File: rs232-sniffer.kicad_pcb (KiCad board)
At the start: 2 copper layers, 110 x 55 mm, 78 parts, among them J1 Stiftleiste 2x8, J2 DB9_Female, J3 DB9_Male, J4 DB9_Female, J5 DB9_Female

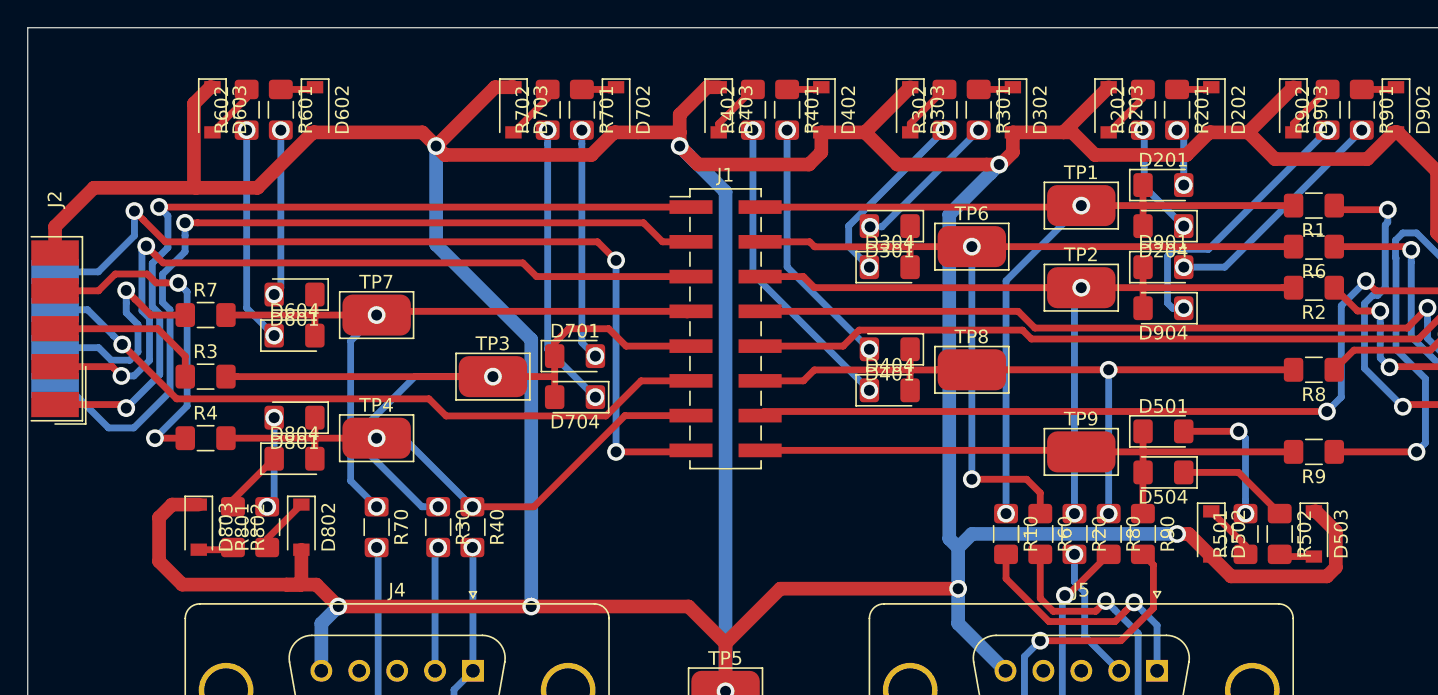
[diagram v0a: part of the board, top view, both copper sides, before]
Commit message: version marius wasinger
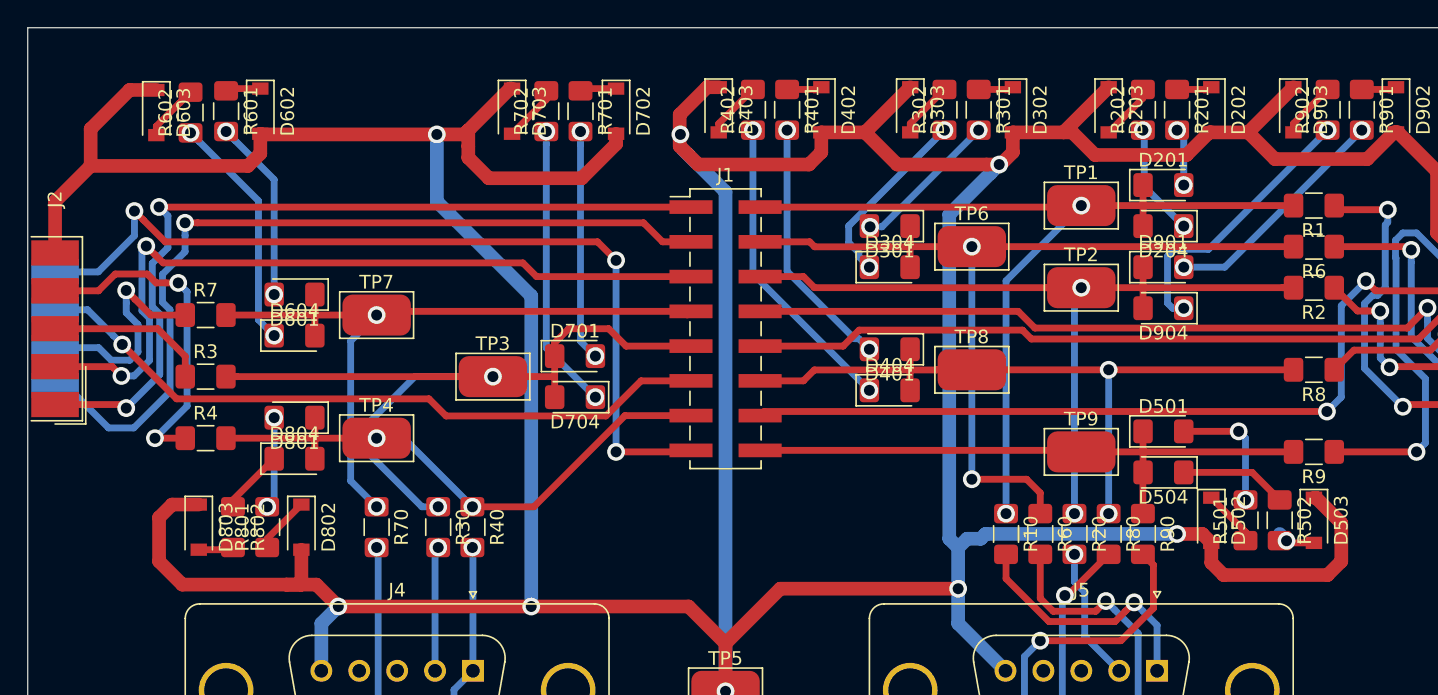
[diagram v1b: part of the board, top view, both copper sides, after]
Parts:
- J2: footprint Connector_Dsub:DSUB-9_Female_EdgeMount_P2.77mm -> rs232-sniffer:DSUB-9_Female_EdgeMount_P2.77mm
- J3: footprint Connector_Dsub:DSUB-9_Male_EdgeMount_P2.77mm -> rs232-sniffer:DSUB-9_Male_EdgeMount_P2.77mm
- J4, J5: footprint Connector_Dsub:DSUB-9_Female_Vertical_P2.77x2.84mm_MountingHoles -> rs232-sniffer:DSUB-9_Female_Vertical_P2.77x2.84mm_MountingHoles
- TP1, TP2, TP3, TP4, TP5, TP6, TP7, TP8, TP9: footprint rs232-sniffer:TestPoint_Pad_5.0x3.0mm -> rs232-sniffer:TestPoint_Pad_5.0x3.0mm_paste
- moved D603 4.10 mm to (68.4, 99.2)
- moved R602 4.10 mm to (70.9, 99.2)
- moved D602 4.00 mm to (76.0, 99.1)
- moved R601 4.00 mm to (73.5, 99.1)
- moved D502 1.00 mm to (145.5, 129.0)
- moved D503 1.00 mm to (153.0, 129.0)
- moved R501 1.00 mm to (148.0, 129.0)
- moved R502 1.00 mm to (150.5, 129.0)
- moved D703 0.14 mm to (94.4, 99.1)
- moved R701 0.14 mm to (99.4, 99.1)
- moved R702 0.14 mm to (96.9, 99.1)
- moved D702 0.10 mm to (102.0, 99.1)
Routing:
- net Net-(D604-Pad1): track 15.8 -> 17.3 mm
- net Net-(D601-Pad2): track 12.2 -> 13.4 mm
- net Net-(D501-Pad2): track 10.2 -> 9.23 mm
- net GND: track 396.0 -> 396.8 mm
- net Net-(D503-Pad2): track 2.57 -> 3.27 mm, vias 0 -> 1

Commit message: wip
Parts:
- removed D201, D301: grün, LED_SMD:LED_1206_3216Metric_Pad1.42x1.75mm_HandSolder
- removed D202, D203, D302, D303, D402, D403, D502, D503, D602, D603, D702, D703, D802, D803, D902, D903: 1N4148W, Diode_SMD:D_SOD-123
- removed D204, D304, D404, D504, D604, D704, D804, D904: rot, LED_SMD:LED_1206_3216Metric_Pad1.42x1.75mm_HandSolder
- removed J4, J5: DB9_Female, rs232-sniffer:DSUB-9_Female_Vertical_P2.77x2.84mm_MountingHoles
- removed R201, R202, R301, R302, R402, R502, R602, R702, R802, R902: 4k7, Resistor_SMD:R_1206_3216Metric_Pad1.42x1.75mm_HandSolder
- removed TP1, TP2, TP3, TP4, TP6, TP7, TP8, TP9: SMD Testpoint, rs232-sniffer:TestPoint_Pad_5.0x3.0mm_paste
- added C2101: 100n, Capacitor_SMD:C_0603_1608Metric, F.Cu at (283.8, 48.0)
- added C2102: 100n, Capacitor_SMD:C_0603_1608Metric, F.Cu at (263.8, 58.0)
- added C2201: 100n, Capacitor_SMD:C_0603_1608Metric, F.Cu at (263.8, 82.3)
- added C2202: 100n, Capacitor_SMD:C_0603_1608Metric, F.Cu at (263.8, 84.8)
- added C2203: 100n, Capacitor_SMD:C_0603_1608Metric, F.Cu at (267.8, 82.3)
- added C2204: 100n, Capacitor_SMD:C_0603_1608Metric, F.Cu at (267.8, 84.8)
- added C2205: 100n, Capacitor_SMD:C_0603_1608Metric, F.Cu at (271.8, 82.3)
- added C2301: 100n, Capacitor_SMD:C_0603_1608Metric, F.Cu at (291.9, 60.6)
- added C2302: 100n, Capacitor_SMD:C_0603_1608Metric, F.Cu at (295.9, 58.1)
- added C2303: 100n, Capacitor_SMD:C_0603_1608Metric, F.Cu at (295.9, 60.6)
- added C2304: 100n, Capacitor_SMD:C_0603_1608Metric, F.Cu at (291.9, 58.1)
- added C2305: 100n, Capacitor_SMD:C_0603_1608Metric, F.Cu at (299.9, 58.1)
- added C2501: 100n, Capacitor_SMD:C_0603_1608Metric, F.Cu at (267.8, 76.6)
- added C2502: 100n, Capacitor_SMD:C_0603_1608Metric, F.Cu at (283.8, 65.1)
- added C2601: 100n, Capacitor_SMD:C_0603_1608Metric, F.Cu at (241.3, 104.7)
- added C2602: 100n, Capacitor_SMD:C_0603_1608Metric, F.Cu at (237.3, 107.2)
- added C2603: 100n, Capacitor_SMD:C_0603_1608Metric, F.Cu at (237.3, 104.7)
- added C2604: 100n, Capacitor_SMD:C_0603_1608Metric, F.Cu at (233.3, 107.2)
- added C2605: 100n, Capacitor_SMD:C_0603_1608Metric, F.Cu at (233.3, 104.7)
- added C2701: 100n, Capacitor_SMD:C_0603_1608Metric, F.Cu at (299.9, 48.0)
- added C2702: 100n, Capacitor_SMD:C_0603_1608Metric, F.Cu at (295.9, 50.5)
- added C2703: 100n, Capacitor_SMD:C_0603_1608Metric, F.Cu at (295.9, 48.0)
- added C2704: 100n, Capacitor_SMD:C_0603_1608Metric, F.Cu at (291.9, 50.5)
- added C2705: 100n, Capacitor_SMD:C_0603_1608Metric, F.Cu at (291.9, 48.0)
- added D1001: red/green, rs232-sniffer:LED_LiteOn_LTST-C195KGJRKT, F.Cu at (298.4, 95.0)
- added D1101: red/green, rs232-sniffer:LED_LiteOn_LTST-C195KGJRKT, F.Cu at (283.6, 105.1)
- added D1301: red/green, rs232-sniffer:LED_LiteOn_LTST-C195KGJRKT, F.Cu at (312.5, 70.4)
- added D1401: red/green, rs232-sniffer:LED_LiteOn_LTST-C195KGJRKT, F.Cu at (299.2, 80.9)
- added D1501: red/green, rs232-sniffer:LED_LiteOn_LTST-C195KGJRKT, F.Cu at (268.8, 95.5)
- added D1601: red/green, rs232-sniffer:LED_LiteOn_LTST-C195KGJRKT, F.Cu at (268.8, 105.1)
- added D1701: red/green, rs232-sniffer:LED_LiteOn_LTST-C195KGJRKT, F.Cu at (312.5, 60.7)
- added D1801: red/green, rs232-sniffer:LED_LiteOn_LTST-C195KGJRKT, F.Cu at (296.9, 71.3)
- added D1901: red/green, rs232-sniffer:LED_LiteOn_LTST-C195KGJRKT, F.Cu at (284.4, 85.4)
- added D2001: red/green, rs232-sniffer:LED_LiteOn_LTST-C195KGJRKT, F.Cu at (312.5, 51.1)
- added H101: MountingHole, MountingHole:MountingHole_4mm, F.Cu at (64.0, 143.0)
- added H102: MountingHole, MountingHole:MountingHole_4mm, F.Cu at (164.0, 143.0)
- added H103: MountingHole, MountingHole:MountingHole_4mm, F.Cu at (64.0, 98.0)
- added H104: MountingHole, MountingHole:MountingHole_4mm, F.Cu at (164.0, 98.0)
- added J2101: USB-C/16p, rs232-sniffer:USB_C_Receptacle_LCSC_C167321, F.Cu at (267.6, 50.9)
- added J2501: USB-C/16p, rs232-sniffer:USB_C_Receptacle_LCSC_C167321, F.Cu at (267.6, 68.0)
- added R1001: 4k7, Resistor_SMD:R_0603_1608Metric, F.Cu at (299.0, 91.9)
- added R107: 100R, Resistor_SMD:R_0603_1608Metric, F.Cu at (223.8, 107.2)
- added R108: 100R, Resistor_SMD:R_0603_1608Metric, F.Cu at (219.8, 109.7)
- added R109: 100R, Resistor_SMD:R_0603_1608Metric, F.Cu at (223.8, 104.7)
- added R110: 100R, Resistor_SMD:R_0603_1608Metric, F.Cu at (219.8, 107.2)
- added R1101: 4k7, Resistor_SMD:R_0603_1608Metric, F.Cu at (284.2, 102.0)
- added R111: 100R, Resistor_SMD:R_0603_1608Metric, F.Cu at (215.8, 109.7)
- added R117: 100R, Resistor_SMD:R_0603_1608Metric, F.Cu at (219.8, 104.7)
- added R118: 100R, Resistor_SMD:R_0603_1608Metric, F.Cu at (215.8, 107.2)
- added R119: 100R, Resistor_SMD:R_0603_1608Metric, F.Cu at (215.8, 104.7)
- added R1301: 4k7, Resistor_SMD:R_0603_1608Metric, F.Cu at (313.1, 67.3)
- added R1401: 4k7, Resistor_SMD:R_0603_1608Metric, F.Cu at (299.8, 77.8)
- added R1501: 4k7, Resistor_SMD:R_0603_1608Metric, F.Cu at (269.4, 92.4)
- added R1601: 4k7, Resistor_SMD:R_0603_1608Metric, F.Cu at (269.4, 102.0)
- added R1701: 4k7, Resistor_SMD:R_0603_1608Metric, F.Cu at (313.1, 57.6)
- added R1801: 4k7, Resistor_SMD:R_0603_1608Metric, F.Cu at (297.5, 68.2)
- added R1901: 4k7, Resistor_SMD:R_0603_1608Metric, F.Cu at (285.0, 82.3)
- added R2001: 4k7, Resistor_SMD:R_0603_1608Metric, F.Cu at (313.1, 48.0)
- added R2101: 100R, Resistor_SMD:R_0603_1608Metric, F.Cu at (267.8, 59.5)
- added R2501: 100R, Resistor_SMD:R_0603_1608Metric, F.Cu at (263.8, 75.1)
- added SW2001: DIP-Switch 8, Button_Switch_SMD:SW_DIP_SPSTx08_Slide_6.7x21.88mm_W8.61mm_P2.54mm_LowProfile, F.Cu at (220.1, 58.6)
- added SW2401: DIP-Switch 8, Button_Switch_SMD:SW_DIP_SPSTx08_Slide_6.7x21.88mm_W8.61mm_P2.54mm_LowProfile, F.Cu at (220.1, 86.9)
- added TP1001: SMD Testpoint, rs232-sniffer:Keystone_5016, F.Cu at (294.1, 92.7)
- added TP102: SMD Testpoint, rs232-sniffer:Keystone_5016, F.Cu at (84.2, 100.8)
- added TP103: SMD Testpoint, rs232-sniffer:Keystone_5016, F.Cu at (120.2, 99.4)
- added TP1101: SMD Testpoint, rs232-sniffer:Keystone_5016, F.Cu at (279.3, 102.8)
- added TP1301: SMD Testpoint, rs232-sniffer:Keystone_5016, F.Cu at (308.2, 68.1)
- added TP1401: SMD Testpoint, rs232-sniffer:Keystone_5016, F.Cu at (294.9, 78.6)
- added TP1501: SMD Testpoint, rs232-sniffer:Keystone_5016, F.Cu at (264.5, 93.2)
- added TP1601: SMD Testpoint, rs232-sniffer:Keystone_5016, F.Cu at (264.5, 102.8)
- added TP1701: SMD Testpoint, rs232-sniffer:Keystone_5016, F.Cu at (308.2, 58.4)
- added TP1801: SMD Testpoint, rs232-sniffer:Keystone_5016, F.Cu at (292.6, 69.0)
- added TP1901: SMD Testpoint, rs232-sniffer:Keystone_5016, F.Cu at (280.1, 83.1)
- added TP2001: SMD Testpoint, rs232-sniffer:Keystone_5016, F.Cu at (308.2, 48.8)
- added TP401: SMD Testpoint, rs232-sniffer:Keystone_5016, F.Cu at (249.6, 105.5)
- added TP501: SMD Testpoint, rs232-sniffer:Keystone_5016, F.Cu at (279.3, 93.2)
- added TP601: SMD Testpoint, rs232-sniffer:Keystone_5016, F.Cu at (308.9, 97.9)
- added TP701: SMD Testpoint, rs232-sniffer:Keystone_5016, F.Cu at (308.9, 88.3)
- added TP801: SMD Testpoint, rs232-sniffer:Keystone_5016, F.Cu at (294.1, 102.4)
- added TP901: SMD Testpoint, rs232-sniffer:Keystone_5016, F.Cu at (309.7, 77.7)
- added U2101: CH340C, Package_SO:SOIC-16_3.9x9.9mm_P1.27mm, F.Cu at (277.6, 52.5)
- added U2501: CH340C, Package_SO:SOIC-16_3.9x9.9mm_P1.27mm, F.Cu at (277.6, 69.6)
- D401, D501, D601, D701, D801, D901: value grün -> red/green; footprint LED_SMD:LED_1206_3216Metric_Pad1.42x1.75mm_HandSolder -> rs232-sniffer:LED_LiteOn_LTST-C195KGJRKT
- J101: renamed from J2; footprint rs232-sniffer:DSUB-9_Female_EdgeMount_P2.77mm -> rs232-sniffer:DSUB-9_Female_Vertical_P2.77x2.84mm_MountingHoles
- R101: renamed from R7; value 0R -> 100R; footprint Resistor_SMD:R_1206_3216Metric_Pad1.42x1.75mm_HandSolder -> Resistor_SMD:R_0603_1608Metric
- R102: renamed from R3; value 0R -> 100R; footprint Resistor_SMD:R_1206_3216Metric_Pad1.42x1.75mm_HandSolder -> Resistor_SMD:R_0603_1608Metric
- R103: renamed from R4; value 0R -> 100R; footprint Resistor_SMD:R_1206_3216Metric_Pad1.42x1.75mm_HandSolder -> Resistor_SMD:R_0603_1608Metric
- R104: renamed from R70; value 0R -> 100R; footprint Resistor_SMD:R_1206_3216Metric_Pad1.42x1.75mm_HandSolder -> Resistor_SMD:R_0603_1608Metric
- R105: renamed from R30; value 0R -> 100R; footprint Resistor_SMD:R_1206_3216Metric_Pad1.42x1.75mm_HandSolder -> Resistor_SMD:R_0603_1608Metric
- R106: renamed from R40; value 0R -> 100R; footprint Resistor_SMD:R_1206_3216Metric_Pad1.42x1.75mm_HandSolder -> Resistor_SMD:R_0603_1608Metric
- R112: renamed from R10; value 0R -> 100R; footprint Resistor_SMD:R_1206_3216Metric_Pad1.42x1.75mm_HandSolder -> Resistor_SMD:R_0603_1608Metric
- R113: renamed from R60; value 0R -> 100R; footprint Resistor_SMD:R_1206_3216Metric_Pad1.42x1.75mm_HandSolder -> Resistor_SMD:R_0603_1608Metric
- R114: renamed from R20; value 0R -> 100R; footprint Resistor_SMD:R_1206_3216Metric_Pad1.42x1.75mm_HandSolder -> Resistor_SMD:R_0603_1608Metric
- R115: renamed from R80; value 0R -> 100R; footprint Resistor_SMD:R_1206_3216Metric_Pad1.42x1.75mm_HandSolder -> Resistor_SMD:R_0603_1608Metric
- R116: renamed from R90; value 0R -> 100R; footprint Resistor_SMD:R_1206_3216Metric_Pad1.42x1.75mm_HandSolder -> Resistor_SMD:R_0603_1608Metric
- R120: renamed from R1; value 0R -> 100R; footprint Resistor_SMD:R_1206_3216Metric_Pad1.42x1.75mm_HandSolder -> Resistor_SMD:R_0603_1608Metric
- R121: renamed from R6; value 0R -> 100R; footprint Resistor_SMD:R_1206_3216Metric_Pad1.42x1.75mm_HandSolder -> Resistor_SMD:R_0603_1608Metric
- R122: renamed from R2; value 0R -> 100R; footprint Resistor_SMD:R_1206_3216Metric_Pad1.42x1.75mm_HandSolder -> Resistor_SMD:R_0603_1608Metric
- R123: renamed from R8; value 0R -> 100R; footprint Resistor_SMD:R_1206_3216Metric_Pad1.42x1.75mm_HandSolder -> Resistor_SMD:R_0603_1608Metric
- R124: renamed from R9; value 0R -> 100R; footprint Resistor_SMD:R_1206_3216Metric_Pad1.42x1.75mm_HandSolder -> Resistor_SMD:R_0603_1608Metric
- R401, R501, R601, R701, R801, R901: footprint Resistor_SMD:R_1206_3216Metric_Pad1.42x1.75mm_HandSolder -> Resistor_SMD:R_0603_1608Metric
- TP101: renamed from TP5; footprint rs232-sniffer:TestPoint_Pad_5.0x3.0mm_paste -> rs232-sniffer:Keystone_5016
- moved R601 240.3 mm to (313.8, 97.1), turned to 0 degrees
- moved D601 235.1 mm to (313.2, 100.2), turned to 0 degrees
- moved R801 224.2 mm to (299.0, 101.6), turned to 0 degrees
- moved D801 220.6 mm to (298.4, 104.6), turned to 0 degrees
- moved D701 215.9 mm to (313.2, 90.6)
- moved R701 214.7 mm to (313.8, 87.5), turned to 0 degrees
- moved D901 174.7 mm to (314.0, 80.0)
- moved R901 159.6 mm to (314.6, 76.9), turned to 0 degrees
- moved D501 144.2 mm to (283.6, 95.5)
- moved R501 141.0 mm to (284.2, 92.4), turned to 0 degrees
- moved R401 140.1 mm to (254.5, 104.7), turned to 0 degrees
- moved D401 132.2 mm to (253.9, 107.7), turned to 0 degrees
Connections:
- D401 pad 1: /ClearToSend -> Net-(D401-Pad1)
- D401 pad 2: Net-(D401-Pad2) -> /LEDs A/Signal1
- D501 pad 1: /RingIndicator -> Net-(D501-Pad1)
- D501 pad 2: Net-(D501-Pad2) -> /LEDs A/Signal2
- D601 pad 1: /ReadyToReceive -> Net-(D601-Pad1)
- D601 pad 2: Net-(D601-Pad2) -> /LEDs A/Signal3
- D701 pad 1: /Sig3 -> Net-(D701-Pad1)
- D701 pad 2: Net-(D701-Pad2) -> /LEDs A/Signal4
- D801 pad 1: /DataTerminalReady -> Net-(D801-Pad1)
- D801 pad 2: Net-(D801-Pad2) -> /LEDs A/Signal6
- D901 pad 1: /ReceiveData -> Net-(D901-Pad1)
- D901 pad 2: Net-(D901-Pad2) -> /LEDs A/Signal7
- J1 pad 1: Net-(J1-Pad1) -> (no net)
- J1 pad 11: /ClearToSend -> (no net)
- J1 pad 14: /ReceiveData -> (no net)
- J1 pad 15: /DataSetReady -> (no net)
- J1 pad 16: /DataCarrierDetect -> (no net)
- J1 pad 2: Net-(J1-Pad2) -> (no net)
- J1 pad 3: Net-(J1-Pad3) -> (no net)
- J1 pad 4: /ReadyToReceive -> (no net)
- J1 pad 5: /Sig3 -> (no net)
- J1 pad 6: Net-(J1-Pad6) -> (no net)
- J1 pad 7: /DataTerminalReady -> (no net)
- J1 pad 8: Net-(J1-Pad8) -> (no net)
- J1 pad 9: /RingIndicator -> (no net)
- J101 pad 1: Net-(J1-Pad1) -> /LEDs A/Signal1
- J101 pad 2: Net-(J1-Pad3) -> /LEDs A/Signal2
- J101 pad 6: Net-(J1-Pad2) -> /LEDs A/Signal6
- J101 pad 8: Net-(J1-Pad6) -> /LEDs A/Signal8
- J101 pad 9: Net-(J1-Pad8) -> /LEDs A/Signal9
- J3 pad 1: Net-(J3-Pad1) -> (no net)
- J3 pad 2: Net-(J3-Pad2) -> (no net)
- J3 pad 6: Net-(J3-Pad6) -> (no net)
- J3 pad 8: Net-(J3-Pad8) -> (no net)
- J3 pad 9: Net-(J3-Pad9) -> (no net)
- R101 pad 2: /ReadyToReceive -> /LEDs A/Signal7
- R102 pad 2: /Sig3 -> /LEDs A/Signal3
- R103 pad 2: /DataTerminalReady -> /LEDs A/Signal4
- R104 pad 1: /ReadyToReceive -> /LEDs A/Signal7
- R104 pad 2: Net-(J4-Pad8) -> (no net)
- R105 pad 1: /Sig3 -> /LEDs A/Signal3
- R105 pad 2: Net-(J4-Pad2) -> (no net)
- R106 pad 1: /DataTerminalReady -> /LEDs A/Signal4
- R106 pad 2: Net-(J4-Pad1) -> (no net)
- R112 pad 1: /DataCarrierDetect -> /LEDs B/Signal1
- R112 pad 2: Net-(J5-Pad1) -> (no net)
- R113 pad 1: /DataSetReady -> /LEDs B/Signal6
- R113 pad 2: Net-(J5-Pad6) -> (no net)
- R114 pad 1: /ReceiveData -> /LEDs B/Signal2
- R114 pad 2: Net-(J5-Pad2) -> (no net)
- R115 pad 1: /ClearToSend -> /LEDs B/Signal8
- R115 pad 2: Net-(J5-Pad8) -> (no net)
- R116 pad 1: /RingIndicator -> /LEDs B/Signal9
- R116 pad 2: Net-(J5-Pad9) -> (no net)
- R120 pad 1: Net-(J3-Pad1) -> (no net)
- R120 pad 2: /DataCarrierDetect -> /LEDs B/Signal1
- R121 pad 1: Net-(J3-Pad6) -> (no net)
- R121 pad 2: /DataSetReady -> /LEDs B/Signal6
- R122 pad 1: Net-(J3-Pad2) -> (no net)
- R122 pad 2: /ReceiveData -> /LEDs B/Signal2
- R123 pad 1: Net-(J3-Pad8) -> (no net)
- R123 pad 2: /ClearToSend -> /LEDs B/Signal8
- R124 pad 1: Net-(J3-Pad9) -> (no net)
- R124 pad 2: /RingIndicator -> /LEDs B/Signal9
- R401 pad 1: Net-(D402-Pad1) -> Net-(D401-Pad1)
- R401 pad 2: Net-(D401-Pad2) -> GND
- R501 pad 1: Net-(D502-Pad1) -> Net-(D501-Pad1)
- R501 pad 2: Net-(D501-Pad2) -> GND
- R601 pad 1: Net-(D602-Pad1) -> Net-(D601-Pad1)
- R601 pad 2: Net-(D601-Pad2) -> GND
- R701 pad 1: Net-(D702-Pad1) -> Net-(D701-Pad1)
- R701 pad 2: Net-(D701-Pad2) -> GND
- R801 pad 1: Net-(D802-Pad1) -> Net-(D801-Pad1)
- R801 pad 2: Net-(D801-Pad2) -> GND
- R901 pad 1: Net-(D902-Pad1) -> Net-(D901-Pad1)
- R901 pad 2: Net-(D901-Pad2) -> GND
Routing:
- net (no net): track 0.00 -> 854.3 mm, vias 0 -> 30
- net /DataCarrierDetect: track 66.8 -> 0.00 mm, vias 2 -> 0
- net /DataSetReady: track 66.1 -> 0.00 mm, vias 2 -> 0
- net Net-(J1-Pad8): track 64.9 -> 0.00 mm, vias 3 -> 0
- net /ReceiveData: track 62.5 -> 0.00 mm, vias 2 -> 0
- net Net-(J1-Pad2): track 61.7 -> 0.00 mm, vias 1 -> 0
- net Net-(J1-Pad1): track 60.9 -> 0.00 mm, vias 2 -> 0
- net /Sig3: track 58.8 -> 0.00 mm, vias 2 -> 0
- net Net-(J1-Pad3): track 57.1 -> 0.00 mm, vias 2 -> 0
- net /ReadyToReceive: track 53.1 -> 0.00 mm, vias 2 -> 0
- net /ClearToSend: track 52.8 -> 0.00 mm, vias 2 -> 0
- net Net-(J1-Pad6): track 50.8 -> 0.00 mm, vias 1 -> 0
- net /RingIndicator: track 45.2 -> 0.00 mm
- net /DataTerminalReady: track 41.8 -> 0.00 mm, vias 2 -> 0
- net Net-(J3-Pad9): track 32.1 -> 0.00 mm, vias 1 -> 0
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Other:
- outline, holes or cut-outs redrawn
- board text added: "TODO: USB-Uart"

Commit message: übergabe an 3ahel
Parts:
- removed D1101, D2001: red/green, rs232-sniffer:LED_LiteOn_LTST-C195KGJRKT
- removed J1: Stiftleiste 2x8, rs232-sniffer:PinHeader_2x08_P2.54mm_Vertical_SMD
- removed J3: DB9_Male, rs232-sniffer:DSUB-9_Male_EdgeMount_P2.77mm
- removed R1101: 4k7, Resistor_SMD:R_0603_1608Metric
- removed R121, R122, R123, R124: 100R, Resistor_SMD:R_0603_1608Metric
- removed TP1101, TP2001: SMD Testpoint, rs232-sniffer:Keystone_5016
- added C101: 10u/16V/X5R, Capacitor_SMD:C_0805_2012Metric, F.Cu at (170.5, 65.5)
- added C102: 10u/16V/X5R, Capacitor_SMD:C_0805_2012Metric, F.Cu at (174.5, 63.0)
- added C2103: 100n, Capacitor_SMD:C_0603_1608Metric, F.Cu at (100.5, 154.2)
- added C2503: 100n, Capacitor_SMD:C_0603_1608Metric, F.Cu at (20.8, 172.5)
- added D101: red/green, htl_smd:LED_LiteOn_LTST-C195KGJRKT, F.Cu at (162.5, 75.2)
- added D102: red/green, htl_smd:LED_LiteOn_LTST-C195KGJRKT, F.Cu at (159.5, 70.0)
- added D1201: red/green, htl_smd:LED_LiteOn_LTST-C195KGJRKT, F.Cu at (121.2, 42.0)
- added D301: red/green, htl_smd:LED_LiteOn_LTST-C195KGJRKT, F.Cu at (53.0, 42.1)
- added J102: Stiftleiste 2x9, Connector_PinHeader_2.54mm:PinHeader_2x09_P2.54mm_Vertical_SMD, F.Cu at (84.5, 52.0)
- added J103: DB9_Male, htl_connectors:DSUB-9_Male_EdgeMount_P2.77mm, F.Cu at (105.5, 42.0)
- added J104: Stiftleiste 2x9, Connector_PinHeader_2.54mm:PinHeader_2x09_P2.54mm_Vertical_SMD, F.Cu at (164.5, 51.5)
- added J2001: Stiftleiste 2x9, Connector_PinHeader_2.54mm:PinHeader_2x09_P2.54mm_Vertical_SMD, F.Cu at (133.0, 149.8)
- added J2002: Buchsenleiste 1x6, horizontal, Connector_PinSocket_2.54mm:PinSocket_1x06_P2.54mm_Horizontal, F.Cu at (85.0, 155.0)
- added J2003: Stiftleiste 2x9, Connector_PinHeader_2.54mm:PinHeader_2x09_P2.54mm_Vertical_SMD, F.Cu at (133.0, 115.5)
- added J2401: Stiftleiste 2x9, Connector_PinHeader_2.54mm:PinHeader_2x09_P2.54mm_Vertical_SMD, F.Cu at (53.2, 168.0)
- added J2402: Buchsenleiste 1x6, horizontal, Connector_PinSocket_2.54mm:PinSocket_1x06_P2.54mm_Horizontal, F.Cu at (72.8, 176.2)
- added J2403: Stiftleiste 2x9, Connector_PinHeader_2.54mm:PinHeader_2x09_P2.54mm_Vertical_SMD, F.Cu at (53.2, 142.8)
- added R1201: 4k7, Resistor_SMD:R_0603_1608Metric, F.Cu at (123.2, 42.0)
- added R2002: 100R, Resistor_SMD:R_0603_1608Metric, F.Cu at (124.5, 142.2)
- added R2003: 100R, Resistor_SMD:R_0603_1608Metric, F.Cu at (124.5, 144.8)
- added R2004: 1k, Resistor_SMD:R_0603_1608Metric, F.Cu at (124.5, 147.2)
- added R2005: 1k, Resistor_SMD:R_0603_1608Metric, F.Cu at (124.5, 149.8)
- added R2006: 1k, Resistor_SMD:R_0603_1608Metric, F.Cu at (124.5, 152.2)
- added R2007: 1k, Resistor_SMD:R_0603_1608Metric, F.Cu at (124.5, 154.8)
- added R2008: 1k, Resistor_SMD:R_0603_1608Metric, F.Cu at (124.5, 157.2)
- added R2009: 1k, Resistor_SMD:R_0603_1608Metric, F.Cu at (124.5, 105.2)
- added R2010: 1k, Resistor_SMD:R_0603_1608Metric, F.Cu at (124.5, 108.0)
- added R2011: 1k, Resistor_SMD:R_0603_1608Metric, F.Cu at (124.5, 110.5)
- added R2012: 100R, Resistor_SMD:R_0603_1608Metric, F.Cu at (124.5, 113.0)
- added R2013: 100R, Resistor_SMD:R_0603_1608Metric, F.Cu at (124.5, 115.5)
- added R2014: 100R, Resistor_SMD:R_0603_1608Metric, F.Cu at (124.5, 118.0)
- added R2015: 100R, Resistor_SMD:R_0603_1608Metric, F.Cu at (124.5, 120.5)
- added R2016: 100R, Resistor_SMD:R_0603_1608Metric, F.Cu at (124.5, 123.0)
- added R2401: 100R, Resistor_SMD:R_0603_1608Metric, F.Cu at (44.8, 157.8)
- added R2402: 100R, Resistor_SMD:R_0603_1608Metric, F.Cu at (44.8, 160.5)
- added R2403: 100R, Resistor_SMD:R_0603_1608Metric, F.Cu at (44.8, 163.0)
- added R2404: 1k, Resistor_SMD:R_0603_1608Metric, F.Cu at (44.8, 165.5)
- added R2405: 1k, Resistor_SMD:R_0603_1608Metric, F.Cu at (44.8, 168.0)
- added R2406: 1k, Resistor_SMD:R_0603_1608Metric, F.Cu at (44.8, 170.5)
- added R2407: 1k, Resistor_SMD:R_0603_1608Metric, F.Cu at (44.8, 173.0)
- added R2408: 1k, Resistor_SMD:R_0603_1608Metric, F.Cu at (44.8, 175.5)
- added R2409: 1k, Resistor_SMD:R_0603_1608Metric, F.Cu at (44.8, 132.5)
- added R2410: 1k, Resistor_SMD:R_0603_1608Metric, F.Cu at (44.8, 135.2)
- added R2411: 1k, Resistor_SMD:R_0603_1608Metric, F.Cu at (44.8, 137.8)
- added R2412: 100R, Resistor_SMD:R_0603_1608Metric, F.Cu at (44.8, 140.2)
- added R2413: 100R, Resistor_SMD:R_0603_1608Metric, F.Cu at (44.8, 142.8)
- added R2414: 100R, Resistor_SMD:R_0603_1608Metric, F.Cu at (44.8, 145.2)
- added R2415: 100R, Resistor_SMD:R_0603_1608Metric, F.Cu at (44.8, 147.8)
- added R2416: 100R, Resistor_SMD:R_0603_1608Metric, F.Cu at (44.8, 150.2)
- added R301: 4k7, Resistor_SMD:R_0603_1608Metric, F.Cu at (55.0, 42.1)
- added SW101: DIP-Switch 8, Button_Switch_SMD:SW_DIP_SPSTx08_Slide_6.7x21.88mm_W8.61mm_P2.54mm_LowProfile, F.Cu at (84.5, 71.0)
- added TP1201: SMD Testpoint, htl_smd:Keystone_5016, F.Cu at (117.8, 42.0)
- added TP301: SMD Testpoint, htl_smd:Keystone_5016, F.Cu at (49.5, 42.1)
- added U101: AMS1117-3.3, Package_TO_SOT_SMD:SOT-223-3_TabPin2, F.Cu at (172.2, 72.2)
- added U2201: MAX3232, Package_SO:SOIC-16_3.9x9.9mm_P1.27mm, F.Cu at (105.0, 120.0)
- added U2301: MAX3232, Package_SO:SOIC-16_3.9x9.9mm_P1.27mm, F.Cu at (115.8, 120.0)
- added U2601: MAX3232, Package_SO:SOIC-16_3.9x9.9mm_P1.27mm, F.Cu at (25.2, 136.8)
- added U2701: MAX3232, Package_SO:SOIC-16_3.9x9.9mm_P1.27mm, F.Cu at (36.0, 136.8)
- D1001, D1301, D1401, D1501, D1601, D1701, D1801, D1901, D401, D501, D601, D701, D801, D901: footprint rs232-sniffer:LED_LiteOn_LTST-C195KGJRKT -> htl_smd:LED_LiteOn_LTST-C195KGJRKT
- J101: footprint rs232-sniffer:DSUB-9_Female_Vertical_P2.77x2.84mm_MountingHoles -> htl_connectors:DSUB-9_Female_EdgeMount_P2.77mm
- J2101, J2501: footprint rs232-sniffer:USB_C_Receptacle_LCSC_C167321 -> htl_connectors:USB_C_Receptacle_LCSC_C167321
- R117, R118: value 100R -> 0R
- R119: value 100R -> 4k7
- R120: value 100R -> 1k
- R2001: value 4k7 -> 100R
- TP1001, TP101, TP102, TP103, TP1301, TP1401, TP1501, TP1601, TP1701, TP1801, TP1901, TP401, TP501, TP601, TP701, TP801, TP901: footprint rs232-sniffer:Keystone_5016 -> htl_smd:Keystone_5016
- moved C2502 284.0 mm to (23.2, 178.2), turned to 180 degrees
- moved C2701 273.9 mm to (39.0, 131.2), turned to 180 degrees
- moved C2703 272.9 mm to (36.0, 131.2), turned to 180 degrees
- moved C2702 271.9 mm to (35.0, 127.0), turned to 90 degrees
- moved U2501 271.6 mm to (26.5, 173.2), turned to 90 degrees
- moved C2704 271.2 mm to (33.0, 131.2)
- moved C2705 266.4 mm to (38.2, 129.5)
- moved D601 264.2 mm to (53.0, 54.8)
- moved TP601 263.0 mm to (49.5, 54.8)
- moved R601 262.3 mm to (55.0, 54.8), turned to 270 degrees
- moved D701 262.1 mm to (53.0, 59.1)
- moved D901 261.3 mm to (53.0, 67.6)
- moved TP701 261.1 mm to (49.5, 59.1)
- moved TP901 260.4 mm to (49.5, 67.6)
- moved R701 260.4 mm to (55.0, 59.1), turned to 270 degrees
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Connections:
- net /UART Hub/USB - UART/~CTS renamed /UART Hub R/USB - UART/~CTS
- net /UART Hub/USB - UART/~RI renamed /UART Hub R/USB - UART/~RI
- net /sheet5F8AD0D9/USB - UART/~CTS renamed /UART Hub L/USB - UART/~CTS
- net /sheet5F8AD0D9/USB - UART/~RI renamed /UART Hub L/USB - UART/~RI
- net Net-(J2101-PadA6) renamed /UART Hub R/USB - UART/D+
- net Net-(J2101-PadA7) renamed /UART Hub R/USB - UART/D-
- net Net-(J2501-PadA6) renamed /UART Hub L/USB - UART/D+
- net Net-(J2501-PadA7) renamed /UART Hub L/USB - UART/D-
- C2101 pad 1: Net-(C2101-Pad1) -> GND
- C2101 pad 2: GND -> Net-(C2101-Pad2)
- C2102 pad 1: GND -> Net-(C2102-Pad1)
- C2102 pad 2: VDD -> GND
- C2201 pad 1: (no net) -> Net-(C2201-Pad1)
- C2201 pad 2: (no net) -> Net-(C2201-Pad2)
- C2202 pad 2: VDD -> +3V3
- C2203 pad 1: (no net) -> Net-(C2203-Pad1)
- C2203 pad 2: (no net) -> Net-(C2203-Pad2)
- C2204 pad 2: (no net) -> Net-(C2204-Pad2)
- C2205 pad 2: (no net) -> Net-(C2205-Pad2)
- C2301 pad 1: (no net) -> Net-(C2301-Pad1)
- C2301 pad 2: (no net) -> Net-(C2301-Pad2)
- C2302 pad 2: VDD -> +3V3
- C2303 pad 1: (no net) -> Net-(C2303-Pad1)
- C2303 pad 2: (no net) -> Net-(C2303-Pad2)
- C2304 pad 2: (no net) -> Net-(C2304-Pad2)
- C2305 pad 2: (no net) -> Net-(C2305-Pad2)
- C2501 pad 1: Net-(C2501-Pad1) -> GND
- C2501 pad 2: GND -> Net-(C2501-Pad2)
- C2502 pad 1: GND -> Net-(C2502-Pad1)
- C2502 pad 2: VDD -> GND
- C2601 pad 1: (no net) -> Net-(C2601-Pad1)
- C2601 pad 2: (no net) -> Net-(C2601-Pad2)
- C2602 pad 2: VDD -> +3V3
- C2603 pad 1: (no net) -> Net-(C2603-Pad1)
- C2603 pad 2: (no net) -> Net-(C2603-Pad2)
- C2604 pad 2: (no net) -> Net-(C2604-Pad2)
- C2605 pad 2: (no net) -> Net-(C2605-Pad2)
- C2701 pad 1: (no net) -> Net-(C2701-Pad1)
- C2701 pad 2: (no net) -> Net-(C2701-Pad2)
- C2702 pad 2: VDD -> +3V3
- C2703 pad 1: (no net) -> Net-(C2703-Pad1)
- C2703 pad 2: (no net) -> Net-(C2703-Pad2)
- C2704 pad 2: (no net) -> Net-(C2704-Pad2)
- C2705 pad 2: (no net) -> Net-(C2705-Pad2)
- D1001 pad 2: /LEDs A/Signal8 -> GND
- D1001 pad 3: /LEDs A/Signal8 -> GND
- D1301 pad 2: /LEDs B/Signal1 -> /LEDs B/Signal2
- D1301 pad 3: /LEDs B/Signal1 -> /LEDs B/Signal2
- D1401 pad 2: /LEDs B/Signal2 -> /LEDs B/Signal3
- D1401 pad 3: /LEDs B/Signal2 -> /LEDs B/Signal3
- D1501 pad 2: /LEDs B/Signal3 -> /LEDs B/Signal4
- D1501 pad 3: /LEDs B/Signal3 -> /LEDs B/Signal4
- D1601 pad 2: /LEDs B/Signal4 -> /LEDs B/Signal6
- D1601 pad 3: /LEDs B/Signal4 -> /LEDs B/Signal6
- D1701 pad 2: /LEDs B/Signal6 -> /LEDs B/Signal7
- D1701 pad 3: /LEDs B/Signal6 -> /LEDs B/Signal7
- D1801 pad 2: /LEDs B/Signal7 -> /LEDs B/Signal8
- D1801 pad 3: /LEDs B/Signal7 -> /LEDs B/Signal8
- D1901 pad 2: /LEDs B/Signal8 -> /LEDs B/Signal9
- D1901 pad 3: /LEDs B/Signal8 -> /LEDs B/Signal9
- D401 pad 2: /LEDs A/Signal1 -> /LEDs A/Signal2
- D401 pad 3: /LEDs A/Signal1 -> /LEDs A/Signal2
- D501 pad 2: /LEDs A/Signal2 -> /LEDs A/Signal3
- D501 pad 3: /LEDs A/Signal2 -> /LEDs A/Signal3
- D601 pad 2: /LEDs A/Signal3 -> /LEDs A/Signal4
- D601 pad 3: /LEDs A/Signal3 -> /LEDs A/Signal4
- D701 pad 2: /LEDs A/Signal4 -> /LEDs A/Signal6
- D701 pad 3: /LEDs A/Signal4 -> /LEDs A/Signal6
- D801 pad 2: /LEDs A/Signal6 -> /LEDs A/Signal7
- D801 pad 3: /LEDs A/Signal6 -> /LEDs A/Signal7
- D901 pad 2: /LEDs A/Signal7 -> /LEDs A/Signal8
- D901 pad 3: /LEDs A/Signal7 -> /LEDs A/Signal8
- J101 pad 3: Net-(J101-Pad3) -> /LEDs A/Signal3
- J101 pad 4: Net-(J101-Pad4) -> /LEDs A/Signal4
- J101 pad 7: Net-(J101-Pad7) -> /LEDs A/Signal7
- J101 pad 9: /LEDs A/Signal9 -> Net-(J101-Pad9)
- J2101 pad A4: VDD -> /UART Hub R/USB-Power
- J2101 pad A9: VDD -> /UART Hub R/USB-Power
- J2101 pad B4: VDD -> /UART Hub R/USB-Power
- J2101 pad B9: VDD -> /UART Hub R/USB-Power
- J2101 pad S1: Net-(J2101-PadS1) -> Net-(C2101-Pad2)
- J2501 pad A4: VDD -> /UART Hub L/USB-Power
- J2501 pad A9: VDD -> /UART Hub L/USB-Power
- J2501 pad B4: VDD -> /UART Hub L/USB-Power
- J2501 pad B9: VDD -> /UART Hub L/USB-Power
- J2501 pad S1: Net-(J2501-PadS1) -> Net-(C2501-Pad2)
- R101 pad 1: Net-(J101-Pad7) -> /LEDs A/Signal3
- R101 pad 2: /LEDs A/Signal7 -> /UART Hub L/RxD
- R102 pad 1: Net-(J101-Pad3) -> /LEDs A/Signal4
- R102 pad 2: /LEDs A/Signal3 -> /UART Hub L/~DCD
- R103 pad 1: Net-(J101-Pad4) -> /LEDs A/Signal4
- R103 pad 2: /LEDs A/Signal4 -> /UART Hub L/~DSR
- R104 pad 2: (no net) -> /UART Hub L/~CTS
- R105 pad 1: /LEDs A/Signal3 -> /UART Hub L/TxD
- R105 pad 2: (no net) -> Net-(R105-Pad2)
- R106 pad 1: /LEDs A/Signal4 -> /UART Hub L/~DTR
- R106 pad 2: (no net) -> Net-(R106-Pad2)
- R107 pad 1: /LEDs A/Signal4 -> /UART Hub L/~DTR
- R107 pad 2: (no net) -> Net-(R107-Pad2)
- R108 pad 1: (no net) -> /UART Hub L/~RTR
- R108 pad 2: (no net) -> Net-(R108-Pad2)
- R109 pad 1: (no net) -> /UART Hub R/TxD
- R109 pad 2: (no net) -> Net-(R109-Pad2)
- R110 pad 1: /UART Hub/~DTR -> /UART Hub R/~DTR
- R110 pad 2: (no net) -> Net-(R110-Pad2)
- R111 pad 1: /UART Hub/~DTR -> /UART Hub R/~RTR
- R111 pad 2: (no net) -> Net-(R111-Pad2)
- R112 pad 1: /LEDs B/Signal1 -> /LEDs B/Signal2
- R112 pad 2: (no net) -> /UART Hub R/RxD
- R113 pad 1: /LEDs B/Signal6 -> /LEDs B/Signal1
- R113 pad 2: (no net) -> /UART Hub R/~DCD
- R114 pad 1: /LEDs B/Signal2 -> /LEDs B/Signal6
- R114 pad 2: (no net) -> /UART Hub R/~DSR
- R115 pad 2: (no net) -> /UART Hub R/~CTS
- R117 pad 1: (no net) -> /UART Hub R/USB-Power
- R117 pad 2: (no net) -> +5V
- R118 pad 1: (no net) -> /UART Hub L/USB-Power
- R118 pad 2: (no net) -> +5V
- R119 pad 1: (no net) -> +5V
- R119 pad 2: (no net) -> Net-(D101-Pad1)
- R120 pad 1: (no net) -> +3V3
- R120 pad 2: /LEDs B/Signal1 -> Net-(D102-Pad1)
- R2001 pad 1: Net-(D2001-Pad1) -> /UART Hub R/USB - UART/TxD
- R2001 pad 2: GND -> Net-(J2001-Pad1)
- SW2001 pad 1: /UART Hub/USB - UART/~DCD -> /UART Hub R/USB - UART/TxD
- SW2001 pad 10: (no net) -> /UART Hub R/UART - RS232 2/UART_Rx2
- SW2001 pad 11: (no net) -> /UART Hub R/UART - RS232 2/UART_Rx1
- SW2001 pad 12: (no net) -> /UART Hub R/UART - RS232 1/UART_Rx2
- SW2001 pad 13: (no net) -> /UART Hub R/UART - RS232 1/UART_Rx1
- SW2001 pad 14: (no net) -> /UART Hub R/UART - RS232 2/UART_Tx1
- SW2001 pad 15: (no net) -> /UART Hub R/UART - RS232 1/UART_Tx2
- SW2001 pad 16: (no net) -> /UART Hub R/UART - RS232 1/UART_Tx1
- SW2001 pad 2: /UART Hub/USB - UART/RxD -> /UART Hub R/USB - UART/~DTR
- SW2001 pad 3: /UART Hub/USB - UART/TxD -> /UART Hub R/USB - UART/~RTR
- SW2001 pad 4: /UART Hub/USB - UART/~DTR -> /UART Hub R/USB - UART/RxD
- SW2001 pad 5: /UART Hub/USB - UART/~DSR -> /UART Hub R/USB - UART/~DCD
- SW2001 pad 6: /UART Hub/USB - UART/~RTR -> /UART Hub R/USB - UART/~DSR
- SW2001 pad 9: (no net) -> +3V3
- SW2401 pad 1: /sheet5F8AD0D9/USB - UART/~DCD -> /UART Hub L/USB - UART/TxD
- SW2401 pad 10: (no net) -> /UART Hub L/UART - RS232 2/UART_Rx2
- SW2401 pad 11: (no net) -> /UART Hub L/UART - RS232 2/UART_Rx1
- SW2401 pad 12: (no net) -> /UART Hub L/UART - RS232 1/UART_Rx2
- SW2401 pad 13: (no net) -> /UART Hub L/UART - RS232 1/UART_Rx1
- SW2401 pad 14: (no net) -> /UART Hub L/UART - RS232 2/UART_Tx1
- SW2401 pad 15: (no net) -> /UART Hub L/UART - RS232 1/UART_Tx2
- SW2401 pad 16: (no net) -> /UART Hub L/UART - RS232 1/UART_Tx1
- SW2401 pad 2: /sheet5F8AD0D9/USB - UART/RxD -> /UART Hub L/USB - UART/~DTR
- SW2401 pad 3: /sheet5F8AD0D9/USB - UART/TxD -> /UART Hub L/USB - UART/~RTR
- SW2401 pad 4: /sheet5F8AD0D9/USB - UART/~DTR -> /UART Hub L/USB - UART/RxD
- SW2401 pad 5: /sheet5F8AD0D9/USB - UART/~DSR -> /UART Hub L/USB - UART/~DCD
- SW2401 pad 6: /sheet5F8AD0D9/USB - UART/~RTR -> /UART Hub L/USB - UART/~DSR
- SW2401 pad 9: (no net) -> +3V3
- TP1001 pad 1: /LEDs A/Signal8 -> GND
- TP1301 pad 1: /LEDs B/Signal1 -> /LEDs B/Signal2
- TP1401 pad 1: /LEDs B/Signal2 -> /LEDs B/Signal3
- TP1501 pad 1: /LEDs B/Signal3 -> /LEDs B/Signal4
- TP1601 pad 1: /LEDs B/Signal4 -> /LEDs B/Signal6
- TP1701 pad 1: /LEDs B/Signal6 -> /LEDs B/Signal7
- TP1801 pad 1: /LEDs B/Signal7 -> /LEDs B/Signal8
- TP1901 pad 1: /LEDs B/Signal8 -> /LEDs B/Signal9
- TP401 pad 1: /LEDs A/Signal1 -> /LEDs A/Signal2
- TP501 pad 1: /LEDs A/Signal2 -> /LEDs A/Signal3
- TP601 pad 1: /LEDs A/Signal3 -> /LEDs A/Signal4
- TP701 pad 1: /LEDs A/Signal4 -> /LEDs A/Signal6
- TP801 pad 1: /LEDs A/Signal6 -> /LEDs A/Signal7
- TP901 pad 1: /LEDs A/Signal7 -> /LEDs A/Signal8
- U2101 pad 10: /UART Hub/USB - UART/~DSR -> /UART Hub R/USB - UART/~DSR
- U2101 pad 12: /UART Hub/USB - UART/~DCD -> /UART Hub R/USB - UART/~DCD
- U2101 pad 13: /UART Hub/USB - UART/~DTR -> /UART Hub R/USB - UART/~DTR
- U2101 pad 14: /UART Hub/USB - UART/~RTR -> /UART Hub R/USB - UART/~RTR
- U2101 pad 16: VDD -> +3V3
- U2101 pad 2: /UART Hub/USB - UART/TxD -> /UART Hub R/USB - UART/TxD
- U2101 pad 3: /UART Hub/USB - UART/RxD -> /UART Hub R/USB - UART/RxD
- U2101 pad 4: Net-(C2101-Pad1) -> Net-(C2102-Pad1)
- U2501 pad 10: /sheet5F8AD0D9/USB - UART/~DSR -> /UART Hub L/USB - UART/~DSR
- U2501 pad 12: /sheet5F8AD0D9/USB - UART/~DCD -> /UART Hub L/USB - UART/~DCD
- U2501 pad 13: /sheet5F8AD0D9/USB - UART/~DTR -> /UART Hub L/USB - UART/~DTR
- U2501 pad 14: /sheet5F8AD0D9/USB - UART/~RTR -> /UART Hub L/USB - UART/~RTR
- U2501 pad 16: VDD -> +3V3
- U2501 pad 2: /sheet5F8AD0D9/USB - UART/TxD -> /UART Hub L/USB - UART/TxD
- U2501 pad 3: /sheet5F8AD0D9/USB - UART/RxD -> /UART Hub L/USB - UART/RxD
- U2501 pad 4: Net-(C2501-Pad1) -> Net-(C2502-Pad1)
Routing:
- net (no net): track 854.3 -> 0.00 mm, vias 30 -> 0
- net GND: track 393.7 -> 111.6 mm, vias 8 -> 12
- net /LEDs A/Signal6: track 0.00 -> 94.1 mm, vias 0 -> 4
- net /LEDs A/Signal8: track 0.00 -> 77.1 mm, vias 0 -> 4
- net /LEDs A/Signal1: track 11.8 -> 80.1 mm, vias 0 -> 3
- net Net-(J1-Pad10): track 62.8 -> 0.00 mm, vias 2 -> 0
- net Net-(J1-Pad13): track 59.3 -> 0.00 mm, vias 1 -> 0
- net /LEDs A/Signal7: track 0.00 -> 59.0 mm, vias 0 -> 2
- net Net-(J1-Pad12): track 56.3 -> 0.00 mm
- net /LEDs A/Signal2: track 24.6 -> 75.4 mm, vias 2 -> 4
- net /LEDs A/Signal4: track 0.00 -> 50.3 mm, vias 0 -> 3
- net /UART Hub R/USB - UART/TxD: track 0.00 -> 47.7 mm
- net /UART Hub L/USB - UART/TxD: track 0.00 -> 47.7 mm
- net /LEDs A/Signal3: track 0.00 -> 47.2 mm, vias 0 -> 2
- net /UART Hub R/USB - UART/~RI: track 0.00 -> 39.6 mm, vias 0 -> 2
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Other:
- board size 110 x 55 mm -> 125 x 150 mm
- net class Default: clearance 0.25 -> 0.15; trace_width 0.25 -> 0.15; via_dia 1.3 -> 0.6; via_drill 0.8 -> 0.3
- rule trace_clearance: 0.25 -> 0.15
- rule trace_min: 0.25 -> 0.15
- rule via_min_drill: 0.8 -> 0.3
- rule via_min_size: 1.3 -> 0.6
- board text removed: "TODO: USB-Uart"
